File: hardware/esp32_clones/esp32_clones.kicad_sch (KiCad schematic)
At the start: 23 parts, among them J2 USB_A, J3 USB_A, J4 USB_A, J5 Micro_SD_Card, J6 Barrel_Jack, J7 DA15_Pins, J9 AudioJack2_Ground

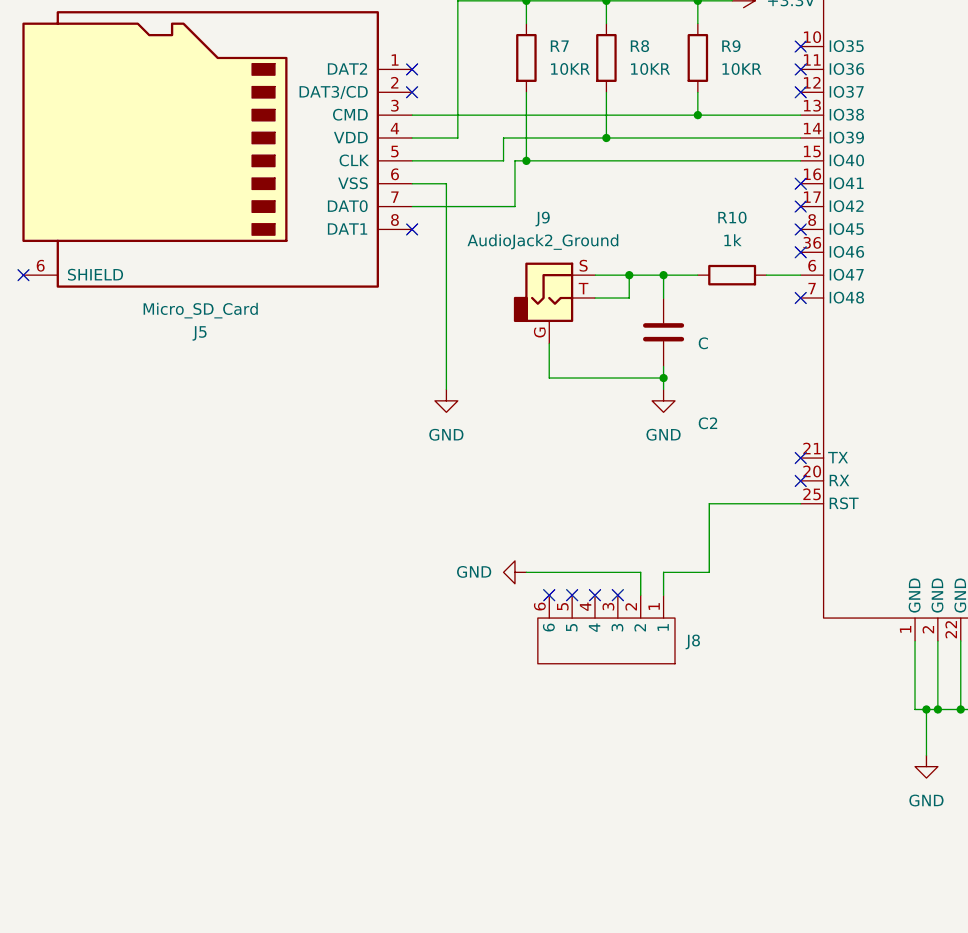
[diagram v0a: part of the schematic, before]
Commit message: Refactor code structure for improved readability and maintainability
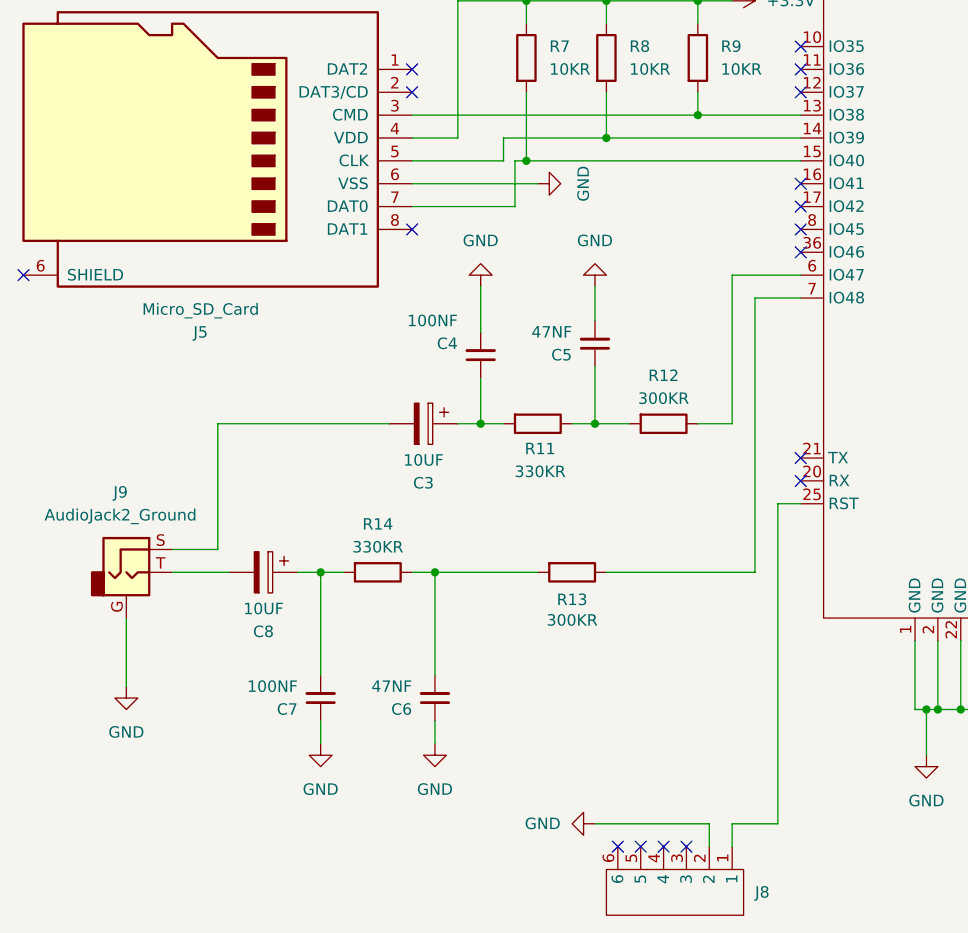
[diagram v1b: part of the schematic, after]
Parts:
- removed C2: C, Capacitor_SMD:C_0805_2012Metric_Pad1.18x1.45mm_HandSolder, symbol Device:C
- removed R10: 1k, Resistor_SMD:R_0805_2012Metric_Pad1.20x1.40mm_HandSolder, symbol Device:R
- added C3, C8: 10UF, Capacitor_SMD:CP_Elec_6.3x3, symbol Device:C_Polarized
- added C4, C7: 100NF, Capacitor_SMD:C_0805_2012Metric_Pad1.18x1.45mm_HandSolder, symbol Device:C_Small
- added C5, C6: 47NF, Capacitor_SMD:C_0805_2012Metric_Pad1.18x1.45mm_HandSolder, symbol Device:C_Small
- added R11, R14: 330KR, Resistor_SMD:R_0805_2012Metric_Pad1.20x1.40mm_HandSolder, symbol Device:R
- added R12, R13: 300KR, Resistor_SMD:R_0805_2012Metric_Pad1.20x1.40mm_HandSolder, symbol Device:R
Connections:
- net GND: now also C4.2, C5.2, C6.1, C7.1
- net at J9.T: now also C8.2; no longer J9.S
- net at U1.6 (IO47): now also R12.1
- net at U1.7 (IO48): now also R13.1
- new net: C3.1, C4.1, R11.2
- new net: C7.2, C8.1, R14.2
- new net: C6.2, R13.2, R14.1
- new net: C5.1, R11.1, R12.2
- new net: C3.2, J9.S
- no-connect marks 33 -> 32
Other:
- moved on the sheet: J8, J9
